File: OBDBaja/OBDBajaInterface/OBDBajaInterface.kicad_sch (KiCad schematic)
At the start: 18 parts, among them J1 Conn_01x02, J10 Conn_01x03, J11 Conn_01x03, J12 Conn_01x03, J13 Conn_01x03, J14 Conn_01x03, J15 Conn_01x03, J16 Conn_01x04, J17 Conn_01x04, J2 Conn_01x05, J3 Conn_01x05, J4 Conn_01x01, J5 Conn_01x01, J6 Conn_01x03, J7 Conn_01x03, J8 Conn_01x03, J9 Conn_01x03, U1 SN65HVD232

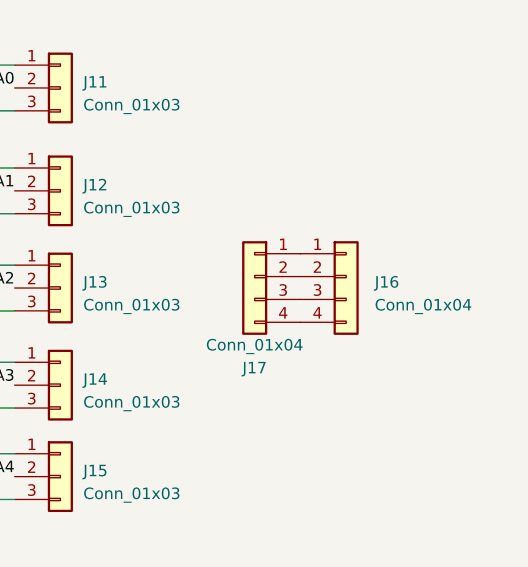
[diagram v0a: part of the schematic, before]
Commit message: Updated OBD Baja file organization
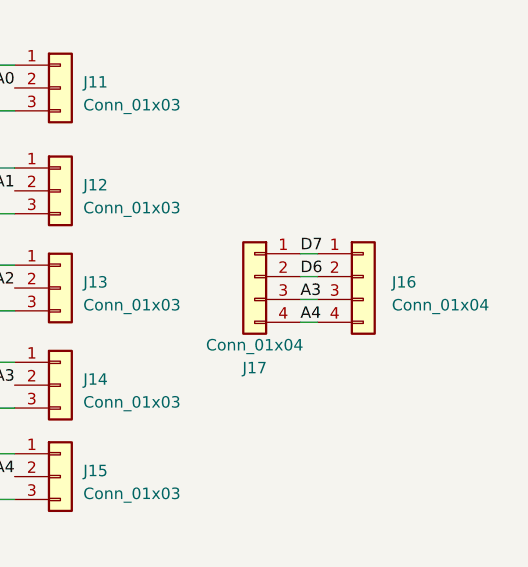
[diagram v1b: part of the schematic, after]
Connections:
- net A3: now also J16.3 (Pin_3), J17.3 (Pin_3)
- net A4: now also J16.4 (Pin_4), J17.4 (Pin_4)
- net D6: now also J16.2 (Pin_2), J17.2 (Pin_2)
- net D7: now also J16.1 (Pin_1), J17.1 (Pin_1)
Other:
- moved on the sheet: J16
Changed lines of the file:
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@@
+    (stroke (width 0) (type default))
+  )
+  (wire (pts (xy 226.06 109.22) (xy 224.155 109.22))
+    (stroke (width 0) (type default))
+  )
+  (wire (pts (xy 226.06 116.84) (xy 224.155 116.84))
     (stroke (width 0) (type default))
   )
@@
     (stroke (width 0) (type default))
   )
+  (wire (pts (xy 226.06 111.76) (xy 224.155 111.76))
+    (stroke (width 0) (type default))
+  )
   (wire (pts (xy 187.96 115.57) (xy 187.96 104.775))
     (stroke (width 0) (type default))
@@
     (stroke (width 0) (type default))
   )
+  (wire (pts (xy 226.06 114.3) (xy 224.155 114.3))
+    (stroke (width 0) (type default))
+  )
   (wire (pts (xy 160.02 104.775) (xy 160.02 93.345))
     (stroke (width 0) (type default))
@@
     (effects (font (size 1.27 1.27)) (justify right bottom))
   )
+  (label "A4" (at 224.155 116.84 0) (fields_autoplaced)
+    (effects (font (size 1.27 1.27)) (justify left bottom))
+  )
   (label "A1" (at 67.945 81.28 180) (fields_autoplaced)
     (effects (font (size 1.27 1.27)) (justify right bottom))
@@
     (effects (font (size 1.27 1.27)) (justify right bottom))
   )
+  (label "D7" (at 224.155 109.22 0) (fields_autoplaced)
+    (effects (font (size 1.27 1.27)) (justify left bottom))
+  )
   (label "D6" (at 164.465 123.825 180) (fields_autoplaced)
     (effects (font (size 1.27 1.27)) (justify right bottom))
@@
     (effects (font (size 1.27 1.27)) (justify right bottom))
   )
+  (label "A3" (at 224.155 114.3 0) (fields_autoplaced)
+    (effects (font (size 1.27 1.27)) (justify left bottom))
+  )
   (label "D5" (at 67.945 63.5 180) (fields_autoplaced)
     (effects (font (size 1.27 1.27)) (justify right bottom))
@@
   (label "A3" (at 192.405 123.825 180) (fields_autoplaced)
     (effects (font (size 1.27 1.27)) (justify right bottom))
+  )
+  (label "D6" (at 224.155 111.76 0) (fields_autoplaced)
+    (effects (font (size 1.27 1.27)) (justify left bottom))
   )
   (label "D3" (at 67.945 58.42 180) (fields_autoplaced)
@@
     )
   )
-  (symbol (lib_id "Connector_Generic:Conn_01x04") (at 229.235 111.76 0) (unit 1)
-    (in_bom yes) (on_board yes) (dnp no) (fields_autoplaced)
-    (property "Reference" "J16" (at 232.41 112.395 0)
-      (effects (font (size 1.27 1.27)) (justify left))
-    )
-    (property "Value" "Conn_01x04" (at 232.41 114.935 0)
-      (effects (font (size 1.27 1.27)) (justify left))
-    )
-    (property "Footprint" "Connector_PinSocket_2.54mm:PinSocket_1x04_P2.54mm_Vertical" (at 229.235 111.76 0)
-      (effects (font (size 1.27 1.27)) hide)
-    )
-    (property "Datasheet" "~" (at 229.235 111.76 0)
-      (effects (font (size 1.27 1.27)) hide)
-    )
+  (symbol (lib_id "Connector_Generic:Conn_01x04") (at 231.14 111.76 0) (unit 1)
+    (in_bom yes) (on_board yes) (dnp no) (fields_autoplaced)
+    (property "Reference" "J16" (at 234.315 112.395 0)
+      (effects (font (size 1.27 1.27)) (justify left))
+    )
+    (property "Value" "Conn_01x04" (at 234.315 114.935 0)
+      (effects (font (size 1.27 1.27)) (justify left))
+    )
+    (property "Footprint" "Connector_PinSocket_2.54mm:PinSocket_1x04_P2.54mm_Vertical" (at 231.14 111.76 0)
+      (effects (font (size 1.27 1.27)) hide)
+    )
+    (property "Datasheet" "~" (at 231.14 111.76 0)
+      (effects (font (size 1.27 1.27)) hide)
+    )
